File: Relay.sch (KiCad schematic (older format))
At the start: 0 parts

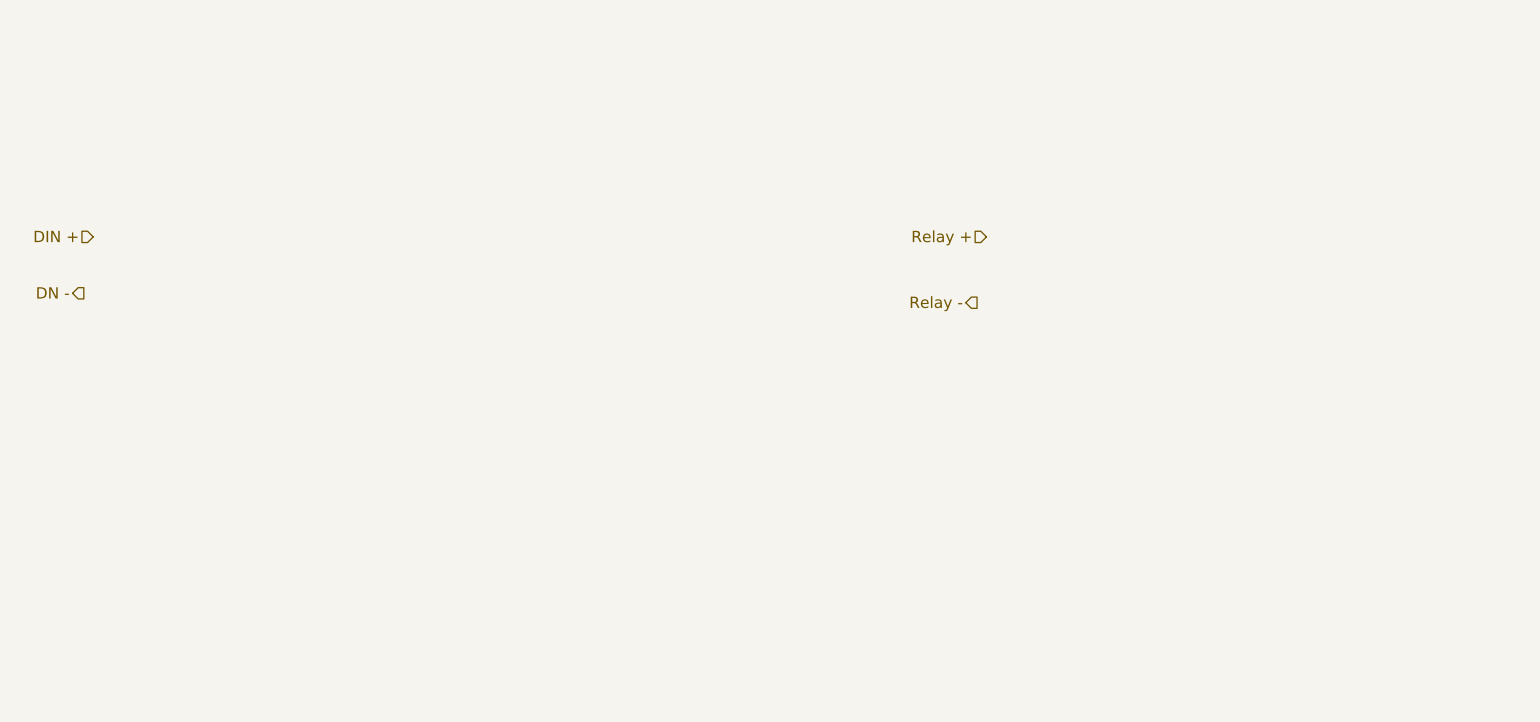
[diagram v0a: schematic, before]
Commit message: Module 3. Unit 5
Relay Block
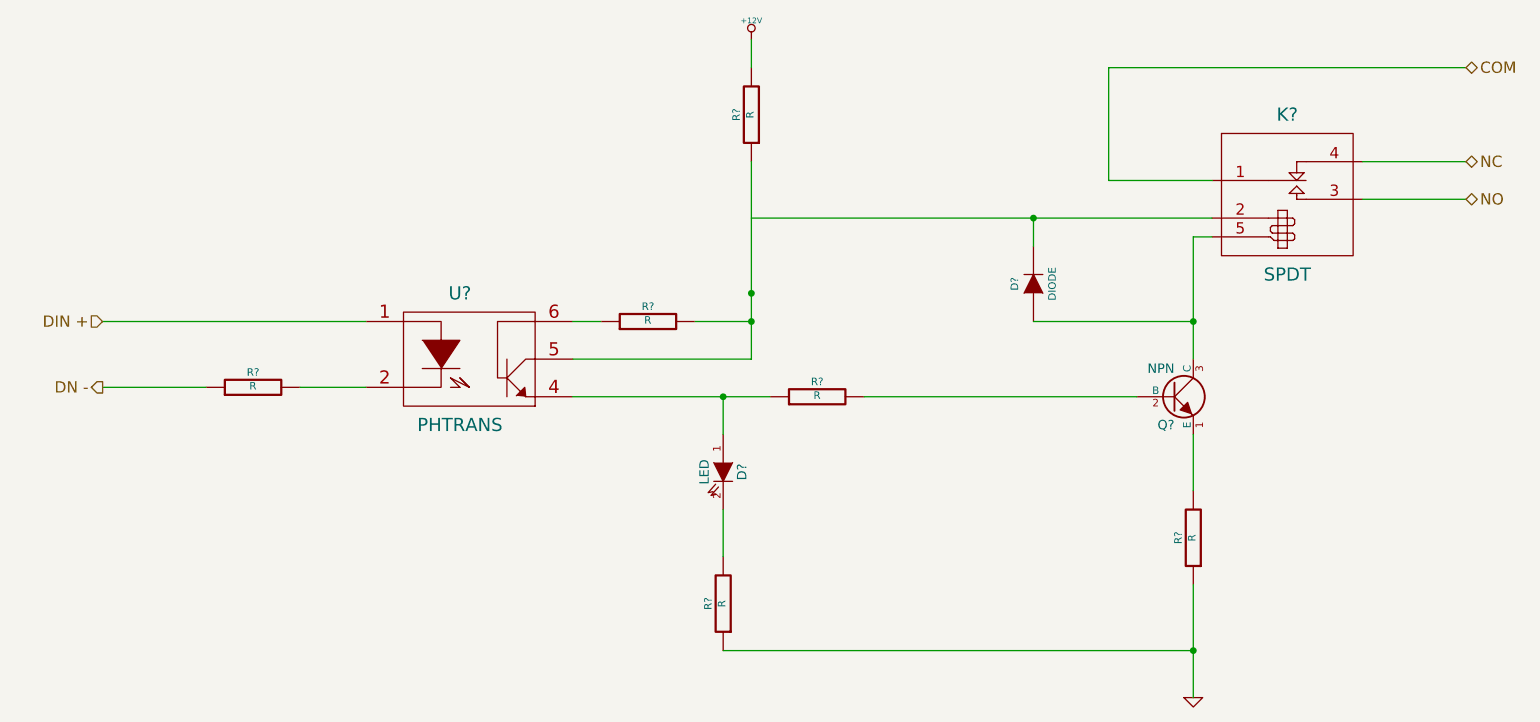
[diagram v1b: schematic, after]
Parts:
- added D?: DIODE, ~, symbol DIODE
- added D?: LED, ~, symbol LED
- added K?: SPDT, ~, symbol SPDT
- added Q?: NPN, ~, symbol NPN
- added R? (x6): R, ~, symbol R
- added U?: PHTRANS, ~, symbol PHTRANS
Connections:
- net labels added: +12V, COM, GND, NC, NO
- net labels removed: Relay +, Relay -
- wire segments 0 -> 25
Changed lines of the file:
@@
 LIBS:contrib
 LIBS:valves
+LIBS:BenchBudEE_Michael_James
 LIBS:BenchBudEE_Michael_James-cache
 EELAYER 27 0
@@
 Comment4 ""
 $EndDescr
-Text HLabel 3150 3450 0    60   Input ~ 0
+Text HLabel 3200 3900 0    60   Input ~ 0
 DIN +
-Text HLabel 3100 3750 0    60   Output ~ 0
+Text HLabel 3200 4250 0    60   Output ~ 0
 DN -
-Text HLabel 7900 3450 0    60   Input ~ 0
-Relay +
-Text HLabel 7850 3800 0    60   Output ~ 0
-Relay -
+Text HLabel 10450 3050 2    60   BiDi ~ 0
+NC
+Text HLabel 10450 3250 2    60   BiDi ~ 0
+NO
+$Comp
+L PHTRANS U?
+U 1 1 52F868D5
+P 5150 4100
+F 0 "U?" H 5100 4450 70  0000 C CNN
+F 1 "PHTRANS" H 5100 3750 70  0000 C CNN
+F 2 "~" H 5150 4100 60  0000 C CNN
+F 3 "~" H 5150 4100 60  0000 C CNN
+	1    5150 4100
+	1    0    0    -1
+$EndComp
+$Comp
+L R R?
+U 1 1 52F868F3
+P 7000 4300
+F 0 "R?" V 7080 4300 40  0000 C CNN
+F 1 "R" V 7007 4301 40  0000 C CNN
+F 2 "~" V 6930 4300 30  0000 C CNN
+F 3 "~" H 7000 4300 30  0000 C CNN
+	1    7000 4300
+	0    -1   -1   0
+$EndComp
+$Comp
+L NPN Q?
+U 1 1 52F86911
+P 8900 4300
+F 0 "Q?" H 8900 4150 50  0000 R CNN
+F 1 "NPN" H 8900 4450 50  0000 R CNN
+F 2 "~" H 8900 4300 60  0000 C CNN
+F 3 "~" H 8900 4300 60  0000 C CNN
+	1    8900 4300
+	1    0    0    -1
+$EndComp
+$Comp
+L LED D?
+U 1 1 52F86920
+P 6500 4700
+F 0 "D?" H 6500 4800 50  0000 C CNN
+F 1 "LED" H 6500 4600 50  0000 C CNN
+F 2 "~" H 6500 4700 60  0000 C CNN
+F 3 "~" H 6500 4700 60  0000 C CNN
+	1    6500 4700
+	0    1    1    0
+$EndComp
+$Comp
+L SPDT K?
+U 1 1 52F84FBF
+P 9500 3100
+F 0 "K?" H 9500 3400 70  0000 C CNN
+F 1 "SPDT" H 9500 2550 70  0000 C CNN
+F 2 "~" H 9500 3100 60  0000 C CNN
+F 3 "~" H 9500 3100 60  0000 C CNN
+	1    9500 3100
+	1    0    0    -1
+$EndComp
+Text HLabel 10450 2550 2    60   BiDi ~ 0
+COM
+Wire Wire Line
+	8550 3150 9100 3150
+Wire Wire Line
+	9900 3050 10450 3050
+Wire Wire Line
+	10450 3250 9900 3250
+Wire Wire Line
+	5700 4300 6750 4300
+Wire Wire Line
+	6650 3350 9100 3350
+Wire Wire Line
+	6650 3050 6650 4100
+$Comp
+L R R?
+U 1 1 52F854DC
+P 9000 5050
+F 0 "R?" V 9080 5050 40  0000 C CNN
+F 1 "R" V 9007 5051 40  0000 C CNN
+F 2 "~" V 8930 5050 30  0000 C CNN
+F 3 "~" H 9000 5050 30  0000 C CNN
+	1    9000 5050
+	-1   0    0    1
+$EndComp
+$Comp
+L GND #PWR?
+U 1 1 52F854EE
+P 9000 5900
+F 0 "#PWR?" H 9000 5900 30  0001 C CNN
+F 1 "GND" H 9000 5830 30  0001 C CNN
+F 2 "" H 9000 5900 60  0000 C CNN
+F 3 "" H 9000 5900 60  0000 C CNN
+	1    9000 5900
+	1    0    0    -1
+$EndComp
+$Comp
+L R R?
+U 1 1 52F85643
+P 6500 5400
+F 0 "R?" V 6580 5400 40  0000 C CNN
+F 1 "R" V 6507 5401 40  0000 C CNN
+F 2 "~" V 6430 5400 30  0000 C CNN
+F 3 "~" H 6500 5400 30  0000 C CNN
+	1    6500 5400
+	-1   0    0    1
+$EndComp
+Wire Wire Line
+	6500 4300 6500 4500
+Connection ~ 6500 4300
+Wire Wire Line
+	6500 4900 6500 5150
+$Comp
+L R R?
+U 1 1 52F85663
+P 6650 2800
+F 0 "R?" V 6730 2800 40  0000 C CNN
+F 1 "R" V 6657 2801 40  0000 C CNN
+F 2 "~" V 6580 2800 30  0000 C CNN
+F 3 "~" H 6650 2800 30  0000 C CNN
+	1    6650 2800
+	-1   0    0    1
+$EndComp
+$Comp
+L +12V #PWR?
+U 1 1 52F8567A
+P 6650 2400
+F 0 "#PWR?" H 6650 2350 20  0001 C CNN
+F 1 "+12V" H 6650 2500 30  0000 C CNN
+F 2 "" H 6650 2400 60  0000 C CNN
+F 3 "" H 6650 2400 60  0000 C CNN
+	1    6650 2400
+	1    0    0    -1
+$EndComp
+Wire Wire Line
+	6650 2400 6650 2550
+Wire Wire Line
+	6500 5650 9000 5650
+Wire Wire Line
+	6650 4100 5700 4100
+Connection ~ 6650 3750
+$Comp
+L R R?
+U 1 1 52F856D2
+P 6100 3900
+F 0 "R?" V 6180 3900 40  0000 C CNN
+F 1 "R" V 6107 3901 40  0000 C CNN
+F 2 "~" V 6030 3900 30  0000 C CNN
+F 3 "~" H 6100 3900 30  0000 C CNN
+	1    6100 3900
+	0    -1   -1   0
+$EndComp
+Wire Wire Line
+	5700 3900 5850 3900
+Wire Wire Line
+	6350 3900 6650 3900
+Connection ~ 6650 3900
+$Comp
+L R R?
+U 1 1 52F8570B
+P 4000 4250
+F 0 "R?" V 4080 4250 40  0000 C CNN
+F 1 "R" V 4007 4251 40  0000 C CNN
+F 2 "~" V 3930 4250 30  0000 C CNN
+F 3 "~" H 4000 4250 30  0000 C CNN
+	1    4000 4250
+	0    -1   -1   0
+$EndComp
+Wire Wire Line
+	4600 3900 3200 3900
+Wire Wire Line
+	3200 4250 3750 4250
+Wire Wire Line
+	4250 4250 4600 4250
+Wire Wire Line
+	8550 3150 8550 2550
+Wire Wire Line
+	8550 2550 10450 2550
+Wire Wire Line
+	7250 4300 8700 4300
+Wire Wire Line
+	9000 4500 9000 4800
+Wire Wire Line
+	9000 5300 9000 5900
+Connection ~ 9000 5650
+Wire Wire Line
+	9100 3450 9000 3450
+Wire Wire Line
+	9000 3450 9000 4100
+$Comp
+L DIODE D?
+U 1 1 52F8597A
+P 8150 3700
+F 0 "D?" H 8150 3800 40  0000 C CNN
+F 1 "DIODE" H 8150 3600 40  0000 C CNN
+F 2 "~" H 8150 3700 60  0000 C CNN
+F 3 "~" H 8150 3700 60  0000 C CNN
+	1    8150 3700
+	0    -1   -1   0
+$EndComp
+Wire Wire Line
+	8150 3350 8150 3500
+Connection ~ 8150 3350
+Wire Wire Line
+	8150 3900 9000 3900
+Connection ~ 9000 3900
 $EndSCHEMATC
